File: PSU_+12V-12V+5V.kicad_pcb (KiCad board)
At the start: 2 copper layers, 118.1 x 74.3 mm, 41 parts, among them J1 Screw_Terminal_01x02, J2 Screw_Terminal_01x02, Q1 BC557, Q2 BC557, Q3 BC547, Q4 BC547, U1 LM317L, U2 LM317L

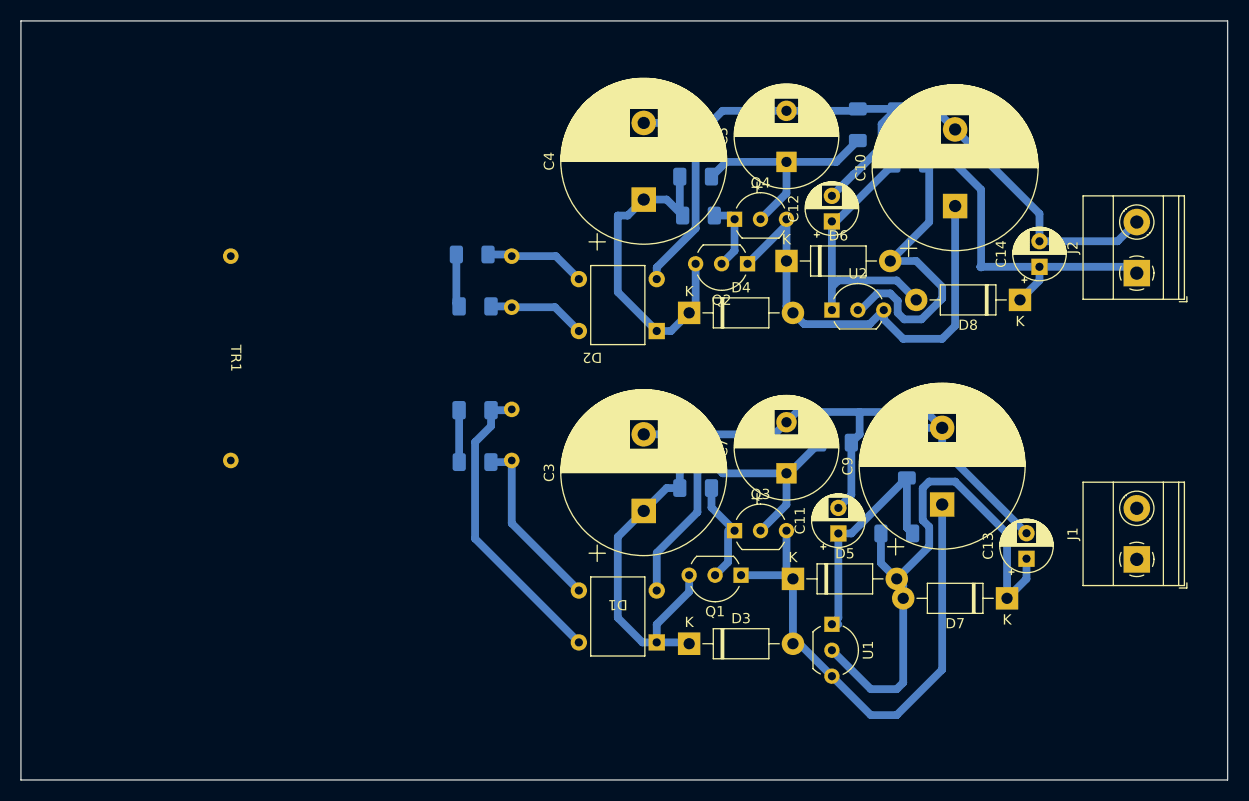
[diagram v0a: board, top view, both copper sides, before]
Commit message: Some shifting
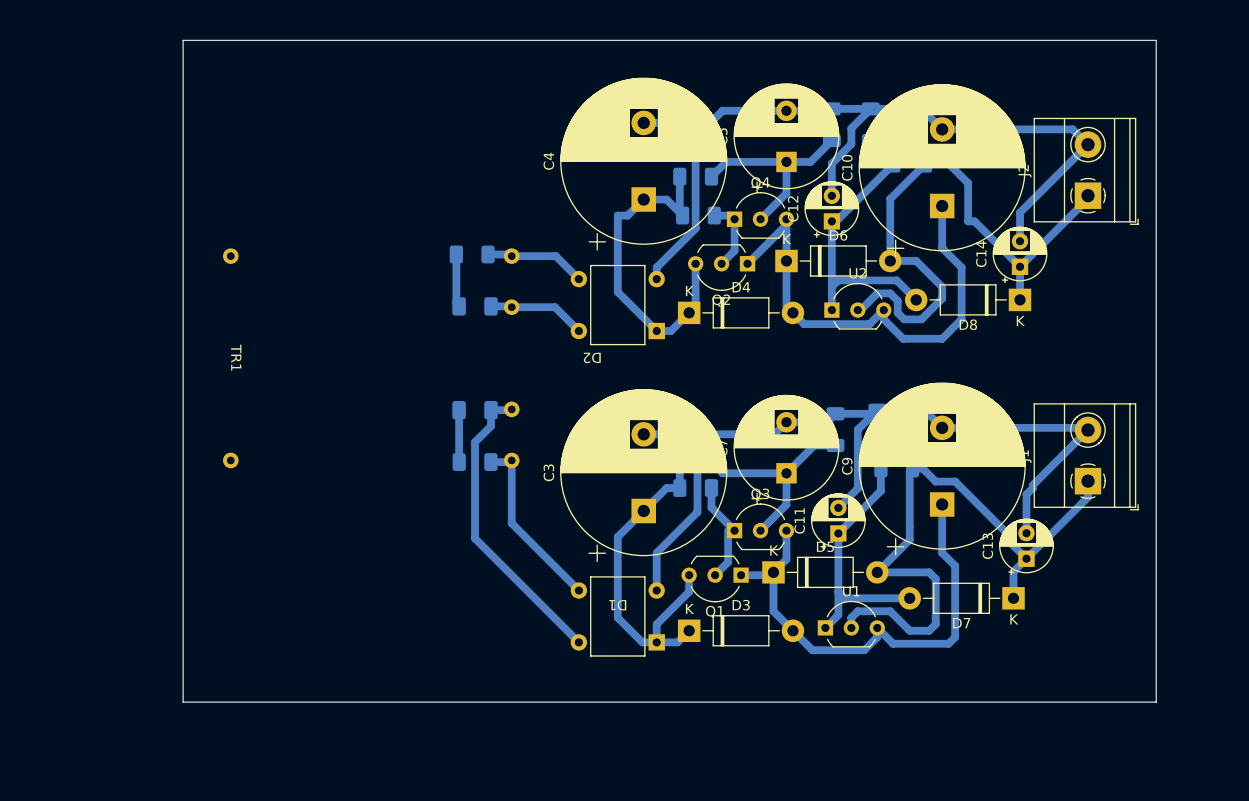
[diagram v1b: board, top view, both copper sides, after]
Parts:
- J1: value Screw_Terminal_01x02 -> PSU12a
- J2: value Screw_Terminal_01x02 -> PSU12b
- moved J1 9.03 mm to (141.3, 83.1)
- moved J2 8.96 mm to (141.3, 55.2)
- moved R11 6.35 mm to (122.6, 81.9), turned to 0 degrees
- moved R12 4.57 mm to (120.7, 77.8)
- moved R14 2.54 mm to (120.0, 48.3)
- moved R6 2.54 mm to (116.2, 48.3)
- moved D5 2.01 mm to (110.5, 92.1)
- moved C14 1.91 mm to (134.6, 62.2)
- moved C10 1.27 mm to (127.0, 56.2)
- moved D3 1.27 mm to (102.2, 97.8)
- moved R9 1.27 mm to (116.6, 78.1), turned to -90 degrees
- moved U1 0.73 mm to (115.6, 97.5), turned to 0 degrees
- moved D7 0.64 mm to (134.0, 94.6)
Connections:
- net Net-(C10-Pad2) renamed /0Vb
- net Net-(C11-Pad2) renamed /0Va
- net Net-(C13-Pad1) renamed /12Va
- net Net-(C14-Pad1) renamed /12Vb
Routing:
- net /0Va: track 75.9 -> 85.9 mm
- net /12Va: track 56.4 -> 62.2 mm
- net /12Vb: track 63.8 -> 58.3 mm
- net Net-(D3-Pad2): track 52.1 -> 46.8 mm
- net Net-(D7-Pad2): track 24.4 -> 27.9 mm
- net Net-(C5-Pad1): track 22.5 -> 19.9 mm
- net Net-(C7-Pad1): track 19.0 -> 20.4 mm
- net Net-(C12-Pad1): track 28.8 -> 29.6 mm
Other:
- board size 118.1 x 74.3 mm -> 95.3 x 64.8 mm
